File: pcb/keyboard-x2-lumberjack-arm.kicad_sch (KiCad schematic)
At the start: 143 parts, among them J1 16-pin USB-C Connector SMD, U1 STM32F103 Bluepill, or MiniF4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, U2 SN74LVC1T45DBV

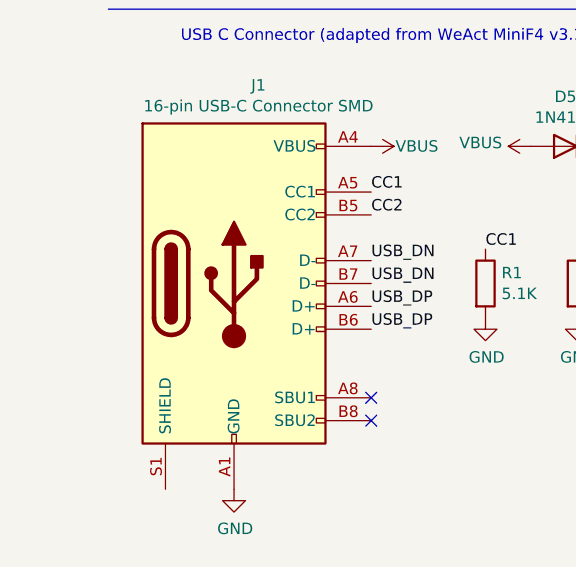
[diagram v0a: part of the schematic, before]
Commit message: Update 20230326
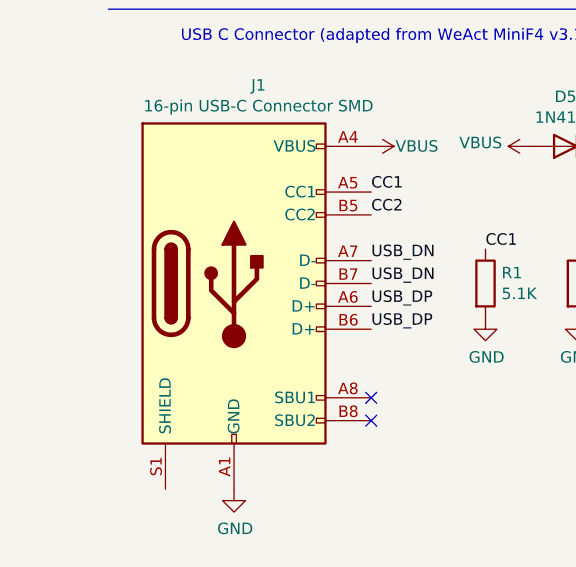
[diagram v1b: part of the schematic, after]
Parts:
- SW_1_1, SW_1_10, SW_1_11, SW_1_12, SW_1_2, SW_1_3, SW_1_4, SW_1_5, SW_1_6, SW_1_7, SW_1_8, SW_1_9, SW_2_1, SW_2_10, SW_2_11, SW_2_12, SW_2_2, SW_2_3, SW_2_4, SW_2_5, SW_2_6, SW_2_7, SW_2_8, SW_2_9, SW_3_1, SW_3_10, SW_3_11, SW_3_12, SW_3_2, SW_3_3, SW_3_4, SW_3_5, SW_3_6, SW_3_7, SW_3_8, SW_3_9, SW_4_1, SW_4_10, SW_4_11, SW_4_12, SW_4_2, SW_4_3, SW_4_4, SW_4_5, SW_4_6, SW_4_7, SW_4_8, SW_4_9, SW_5_1, SW_5_10, SW_5_11, SW_5_12, SW_5_2, SW_5_3, SW_5_4, SW_5_5, SW_5_6, SW_5_7, SW_5_8, SW_5_9: footprint ProjectLocal:SW_MX_PG1350_NoLed -> Library:CherryMX_Choc_Hotswap Single Side
